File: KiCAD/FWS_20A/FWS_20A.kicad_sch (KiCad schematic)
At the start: 85 parts, among them J1 pwr, J2 Conn_01x02_Pin, J3 Conn_01x09_Socket, J4 Conn_01x02_Pin, J5 sense, Q1 DMN32D2LDF, Q6 DMN32D2LDF, SW2 SW_Push, U1 XMSM0L1306SRGER, U11 FCX495, U12 ADS1015IDGS, U2 FDMS8333L, U3 FDMS8333L, U4 LM5109BSD, U5 LM5109BSD, U6 L78L33_SO8, U7 FDMS8333L, U8 FDMS8333L

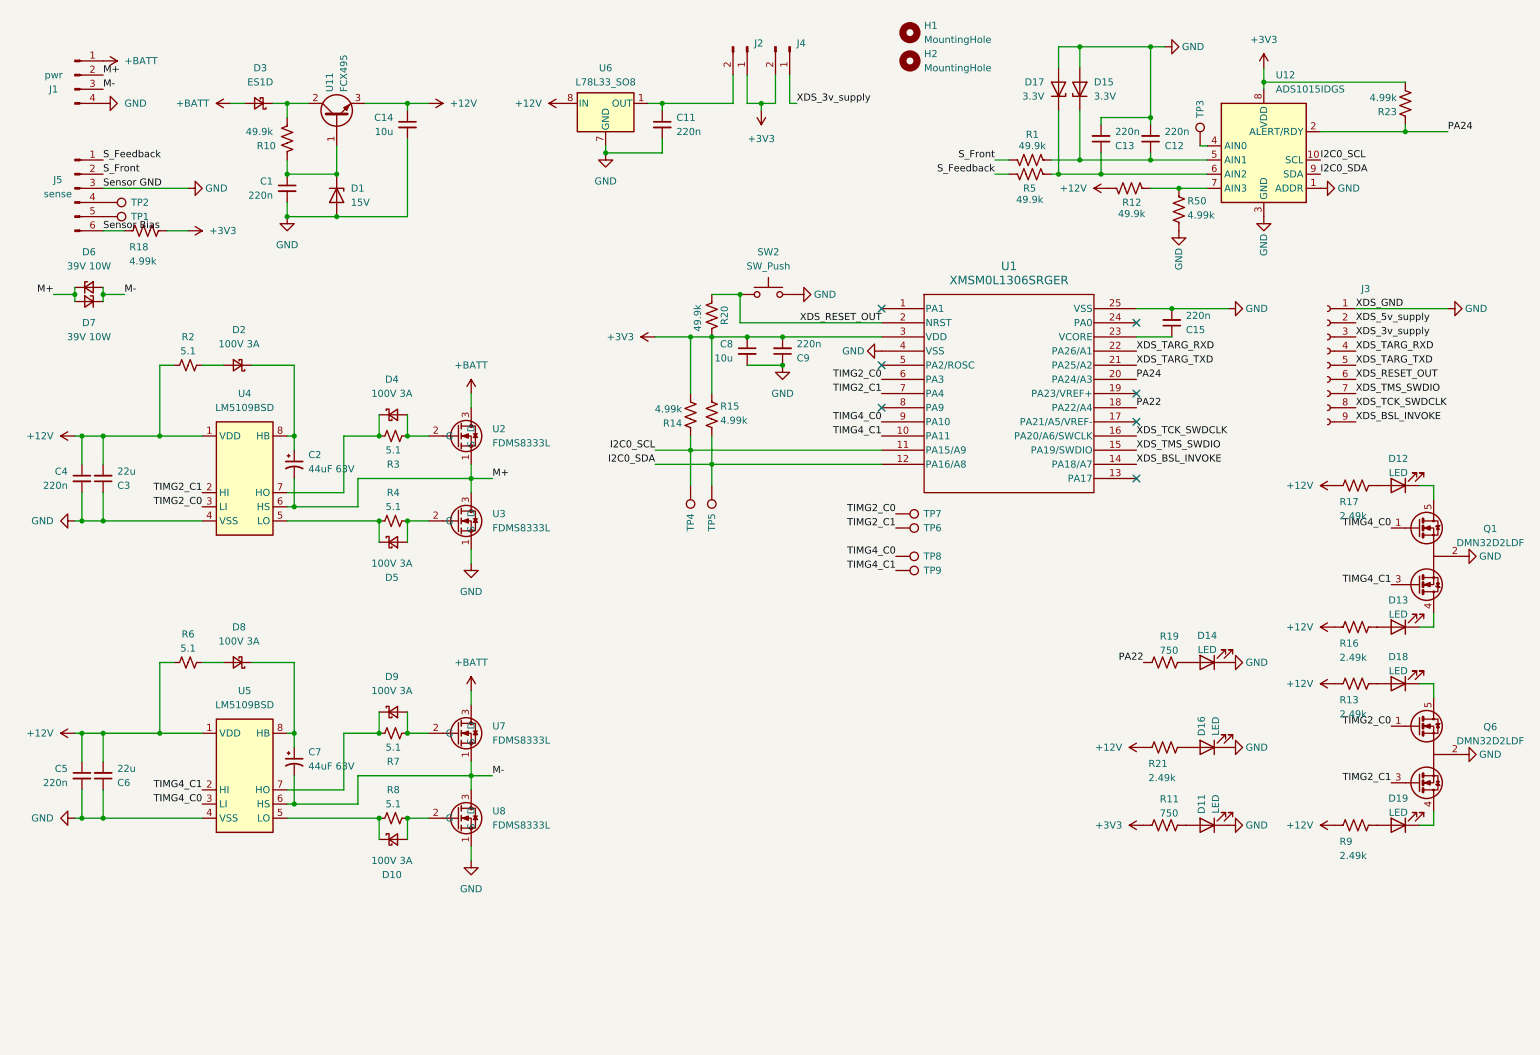
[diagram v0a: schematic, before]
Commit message: cleaned up a bit
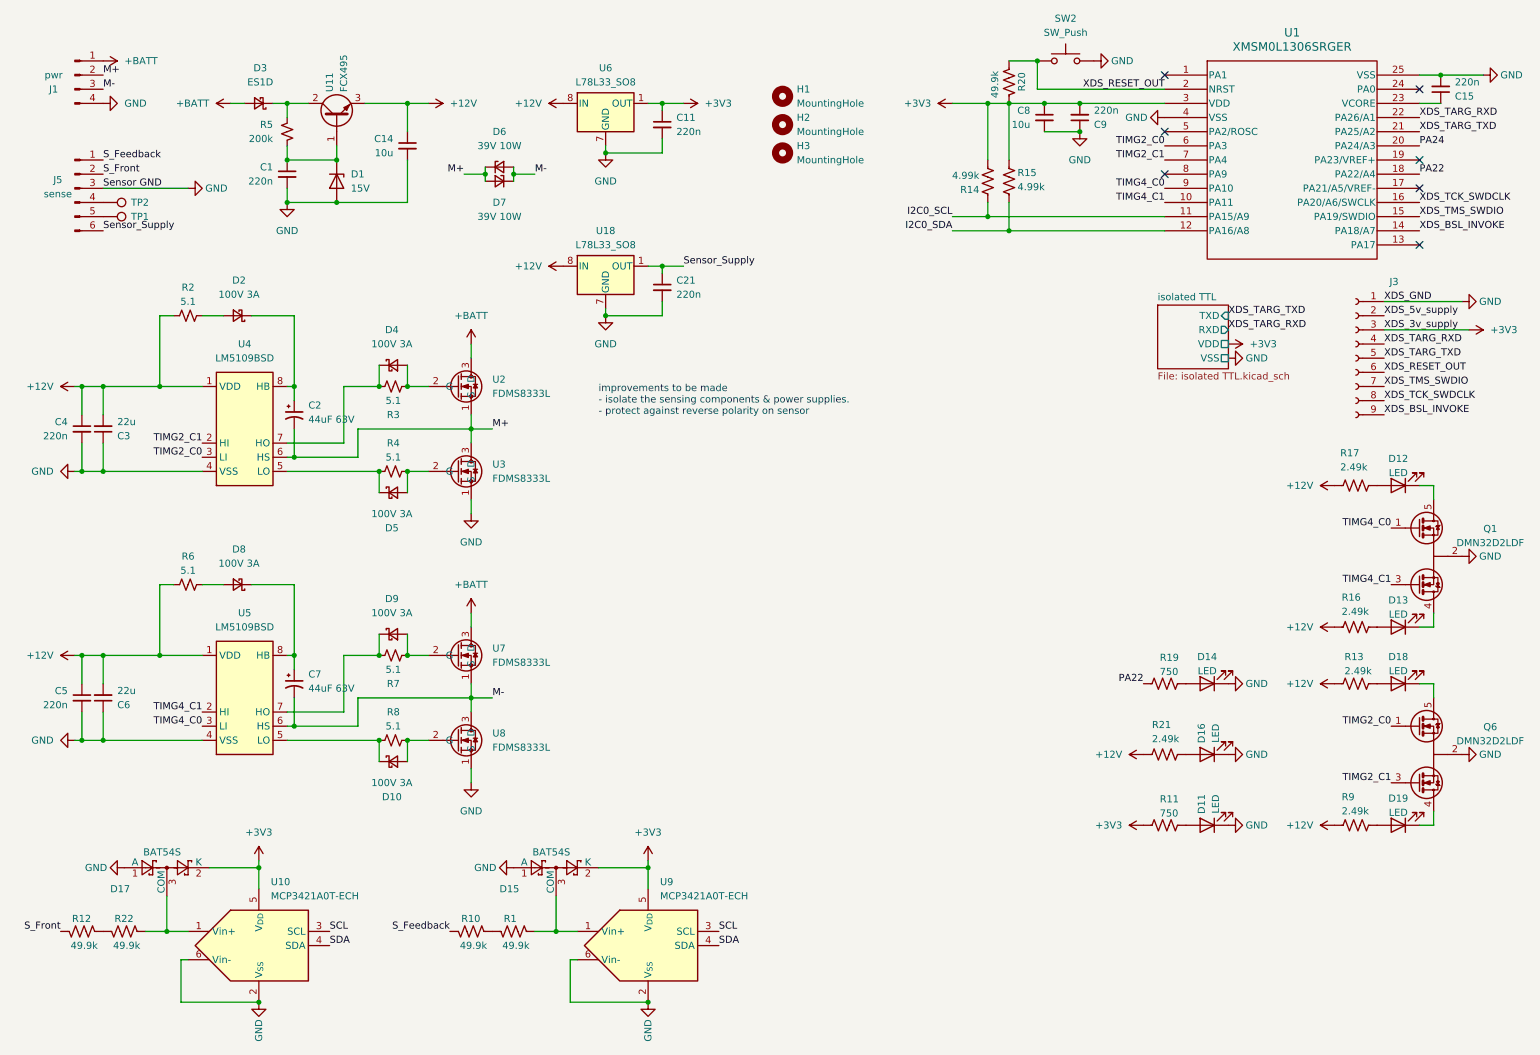
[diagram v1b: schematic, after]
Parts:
- removed C12, C13: 220n, Capacitor_SMD:C_1206_3216Metric_Pad1.33x1.80mm_HandSolder, symbol Device:C_Small
- removed D15, D17: 3.3V, Diode_SMD:D_SOD-323, symbol Device:D_Zener
- removed J2, J4: Conn_01x02_Pin, Connector_PinHeader_2.54mm:PinHeader_1x02_P2.54mm_Vertical, symbol Connector:Conn_01x02_Pin
- removed R18, R23, R50: 4.99k, Resistor_SMD:R_1206_3216Metric_Pad1.30x1.75mm_HandSolder, symbol Device:R_US
- removed R5: 49.9k, Resistor_SMD:R_1206_3216Metric_Pad1.30x1.75mm_HandSolder, symbol Device:R_US
- removed TP3: TestPoint, TestPoint:TestPoint_Loop_D2.50mm_Drill1.0mm_LowProfile, symbol Connector:TestPoint
- removed TP4, TP5, TP6, TP7, TP8, TP9: TestPoint, TestPoint:TestPoint_Pad_D2.0mm, symbol Connector:TestPoint
- removed U12: ADS1015IDGS, Package_SO:TSSOP-10_3x3mm_P0.5mm, symbol Analog_ADC:ADS1015IDGS
- added C21: 220n, Capacitor_SMD:C_1206_3216Metric_Pad1.33x1.80mm_HandSolder, symbol Device:C_Small
- added D15, D17: BAT54S, Package_TO_SOT_SMD:SOT-23-3, symbol Diode:BAT54S
- added H3: MountingHole, MountingHole:MountingHole_2.2mm_M2_DIN965, symbol Mechanical:MountingHole
- added R22: 49.9k, Resistor_SMD:R_1206_3216Metric_Pad1.30x1.75mm_HandSolder, symbol Device:R_US
- added R5: 200k, Resistor_SMD:R_0805_2012Metric_Pad1.20x1.40mm_HandSolder, symbol Device:R_Small_US
- added U10, U9: MCP3421A0T-ECH, Package_TO_SOT_SMD:SOT-23-6, symbol Analog_ADC:MCP3421A0T-ECH
- added U18: L78L33_SO8, Package_SO:SOIC-8_3.9x4.9mm_P1.27mm, symbol Regulator_Linear:L78L33_SO8
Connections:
- net XDS_3v_supply is gone; now on net +3V3: J3.3 (Pin_3)
- net +12V: now also U18.8 (IN); no longer R12.2
- net +3V3: now also C11.1, U6.1 (OUT), D15.2 (K), D17.2 (K), U10.5 (V_{DD}), U9.5 (V_{DD})
- net GND: now also C21.2, D15.1 (A), D17.1 (A), U10.2 (V_{SS}), U10.6 (Vin-), U18.2 (GND), U18.3 (GND), U18.6 (GND), U18.7 (GND), U9.2 (V_{SS}), U9.6 (Vin-)
- net S_Feedback: now also R10.2
- net S_Front: now also R12.2; no longer R1.1
- net at R1.2: now also R10.1
- net at R12.1: now also R22.2
- net at C1.1, D1.1 (K), U11.1: now also R5.1; no longer R10.1
- net at D3.1 (K), U11.2: now also R5.2; no longer R10.2
- net Sensor Bias renamed Sensor_Supply
- net Sensor_Supply: now also C21.1, U18.1 (OUT)
- new net: D17.3 (COM), R22.1, U10.1 (Vin+)
- new net: D15.3 (COM), R1.1, U9.1 (Vin+)
- new net SCL: U10.3 (SCL), U9.3 (SCL)
- new net SDA: U10.4 (SDA), U9.4 (SDA)
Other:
- added sheet isolated TTL (isolated TTL.kicad_sch)
- note added: "improvements to be made - isolate the sensing components & power supplies. - protect against reverse polarity on sensor"
- moved on the sheet: C1, C14, C15, C2, C3, C4, C5, C6, C7, C8, C9, D1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
